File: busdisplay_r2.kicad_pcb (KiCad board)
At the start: 2 copper layers, 35 x 53 mm, 27 parts, among them J1 Hex/Dec, J2 ICSP, J3 Input, J4 Power, Q1 AO3401A, Q2 AO3401A, Q3 AO3401A, U1 PIC16F570-ISO, U2 74HCT245

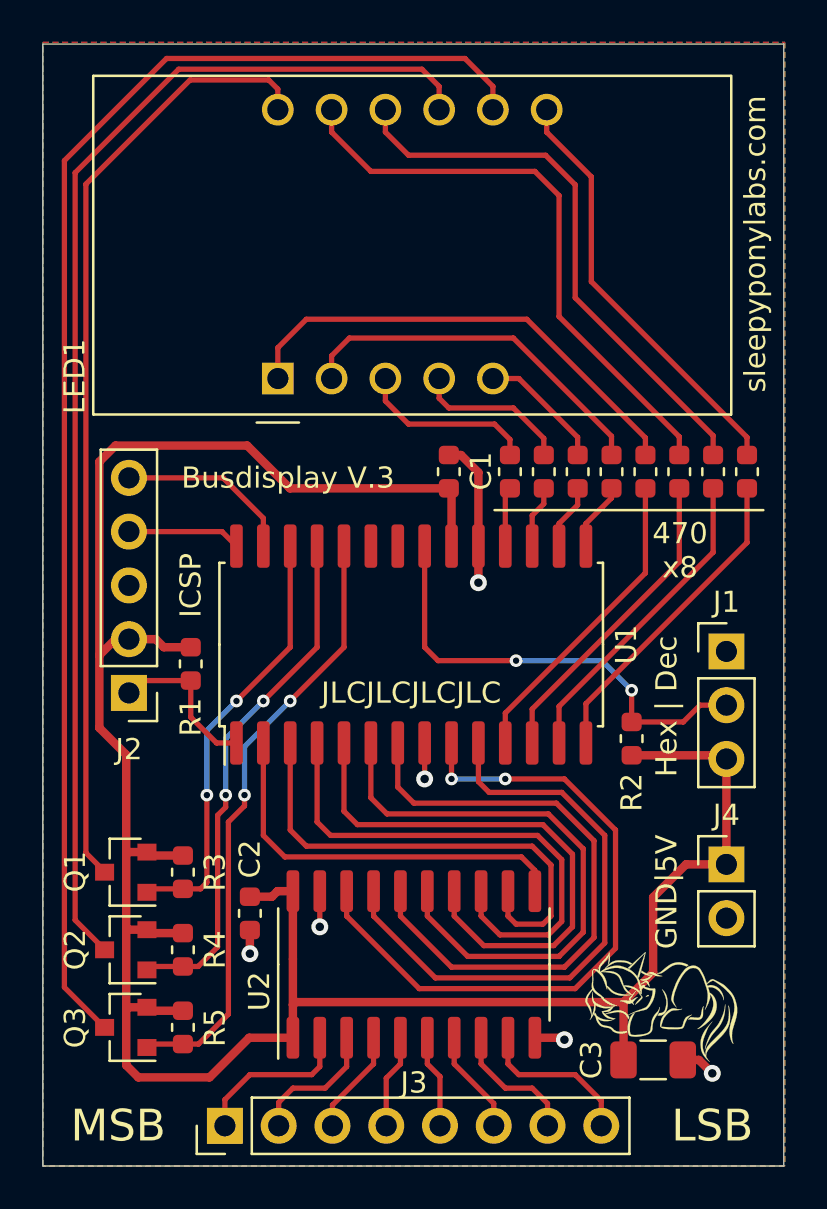
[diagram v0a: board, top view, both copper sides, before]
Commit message: Add firmware, gerbers and ibom
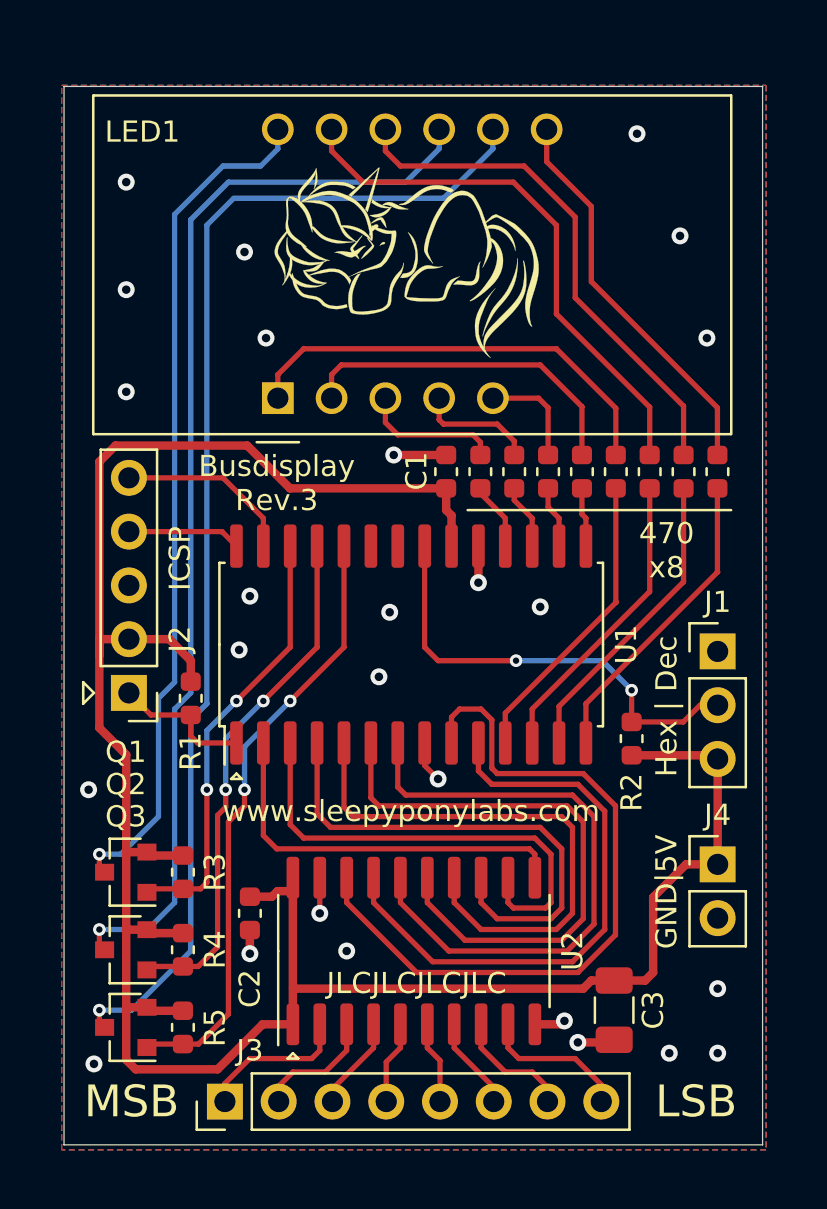
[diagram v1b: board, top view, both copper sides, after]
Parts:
- removed the G*** at (62.7, 75.0)
- added G***: LOGO, sleepyLogo:sleepylogo_15mm, F.Cu at (50.8, 39.6)
- moved C3 2.99 mm to (60.4, 75.4), turned to 270 degrees
- moved R1 1.63 mm to (40.4, 60.7)
- moved R7 1.40 mm to (65.3, 50.0)
- moved R9 1.40 mm to (58.9, 50.0)
- moved R10 1.40 mm to (60.5, 50.0)
- moved R12 1.40 mm to (57.3, 50.0)
- moved R13 1.40 mm to (54.1, 50.0)
- moved R6 1.40 mm to (62.1, 50.0)
- moved R8 1.40 mm to (55.7, 50.0)
- moved R11 1.40 mm to (63.7, 50.0)
- moved J3 1.14 mm to (42.0, 79.8)
- moved LED1 0.93 mm to (44.5, 46.2)
- moved U2 0.63 mm to (50.9, 72.6)
- moved J1 0.41 mm to (65.3, 58.5)
- moved J4 0.41 mm to (65.3, 68.6)
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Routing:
- net Net-(LED1-Pad8): track 65.6 -> 56.9 mm, vias 0 -> 1
- net Net-(LED1-Pad9): track 57.9 -> 51.8 mm, vias 0 -> 1
- net Net-(LED1-Pad12): track 45.1 -> 40.3 mm, vias 0 -> 1
- net +5V: track 118.3 -> 115.2 mm
- net GND: track 14.5 -> 12.2 mm, vias 6 -> 26
- net BUF7: track 32.1 -> 34.4 mm, vias 2 -> 0
- net Net-(LED1-Pad11): track 27.7 -> 25.8 mm
- net Net-(LED1-Pad10): track 26.5 -> 24.6 mm
- net Net-(LED1-Pad4): track 7.45 -> 5.64 mm
- net Net-(LED1-Pad3): track 8.43 -> 6.63 mm
- net Net-(LED1-Pad1): track 22.5 -> 21.0 mm
- net Net-(LED1-Pad7): track 20.2 -> 18.7 mm
- net Net-(LED1-Pad2): track 17.5 -> 16.2 mm
- net Net-(LED1-Pad5): track 6.07 -> 5.03 mm
- net ~MCLR: track 7.55 -> 6.64 mm
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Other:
- board size 35 x 53 mm -> 33 x 50 mm
- board text added: "Busdisplay Rev.3"
- board text added: "www.sleepyponylabs.com"
- board text removed: "Busdisplay V.3"
- board text removed: "sleepyponylabs.com"
